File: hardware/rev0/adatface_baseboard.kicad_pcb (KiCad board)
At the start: 4 copper layers, 121.3 x 111.6 mm, 90 parts, among them J1 Conn_01x06_Male, J2 Conn_02x32_Odd_Even, J3 Conn_02x32_Odd_Even, J4 Connector_USB_C_Receptacle_US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, J5 Connector_USB_C_Receptacle_US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, J6 Conn_01x06_Male, J7 Conn_01x26_Male, J8 Conn_01x01_Male, J9 Conn_01x01_Male, U1 PLR135_T8, U2 PLR135_T8, U3 PLR135_T8, U4 PLR135_T8, U5 USB3320, U6 USB3320, U7 ME6212C18M5G

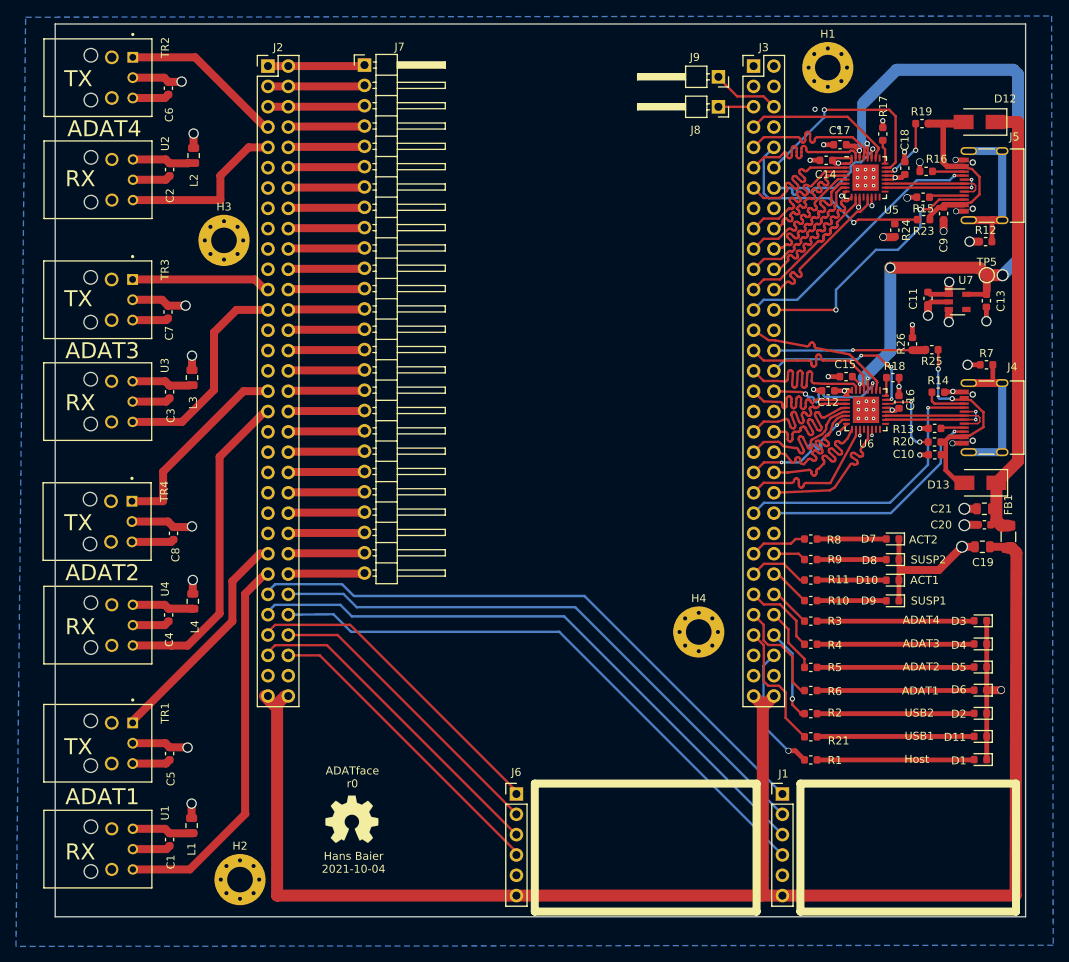
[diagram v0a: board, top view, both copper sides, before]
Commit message: fix DRC errors
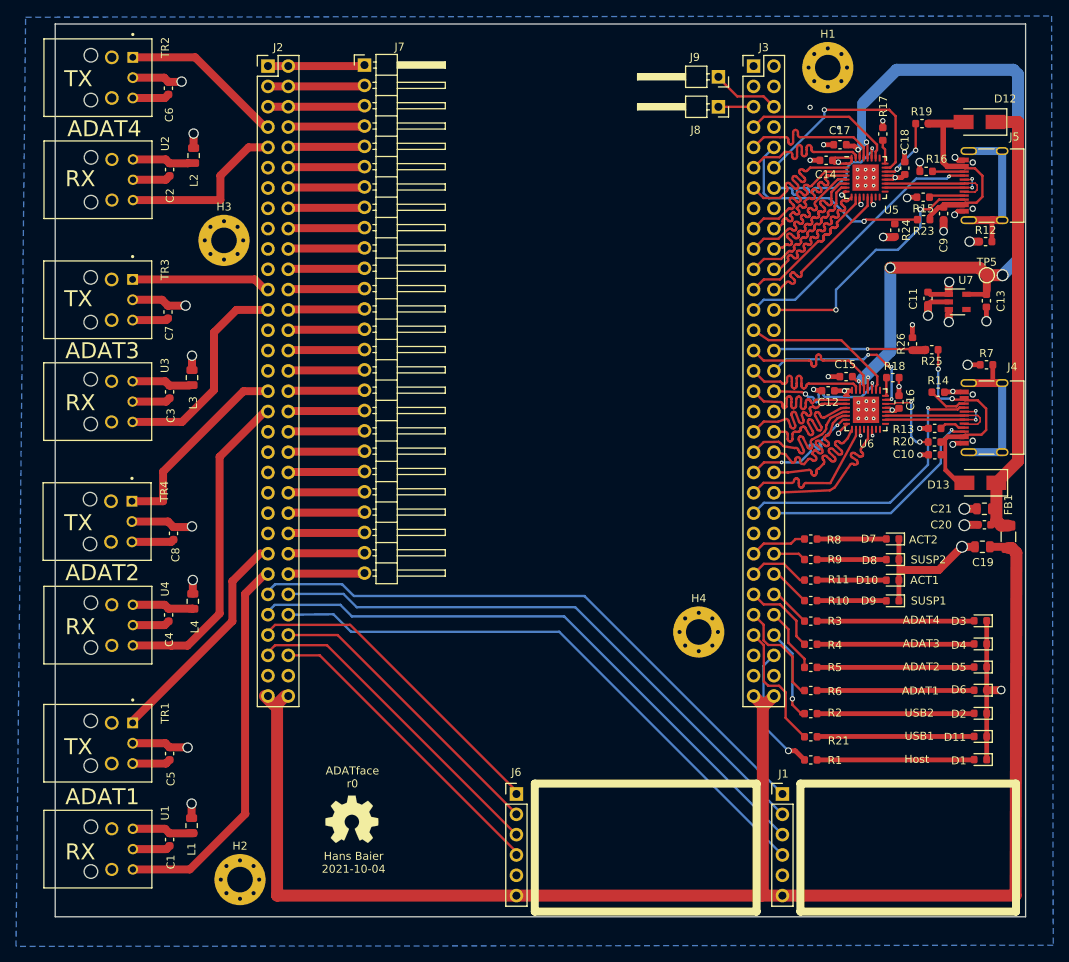
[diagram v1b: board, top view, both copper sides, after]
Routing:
- net /USB1_DIR: track 23.6 -> 18.9 mm
- net GND: track 137.5 -> 141.7 mm
- net /USB1_VBUS: track 34.1 -> 35.8 mm
- net /USB1_D-: track 13.4 -> 14.6 mm
- net /USB2_VBUS: track 36.4 -> 37.5 mm
- net +1V8: track 104.8 -> 105.7 mm
- net /USB2_D-: track 13.4 -> 14.0 mm
- net /USB1_SBU2: track 29.3 -> 29.9 mm
